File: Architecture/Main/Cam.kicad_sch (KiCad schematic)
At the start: 4 parts, among them J2 Conn_01x02, Q3 NMOS

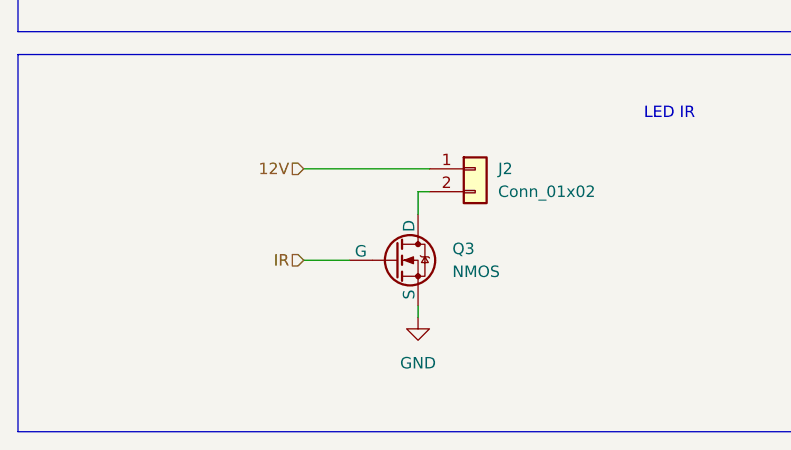
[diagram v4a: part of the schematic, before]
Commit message: Update_She
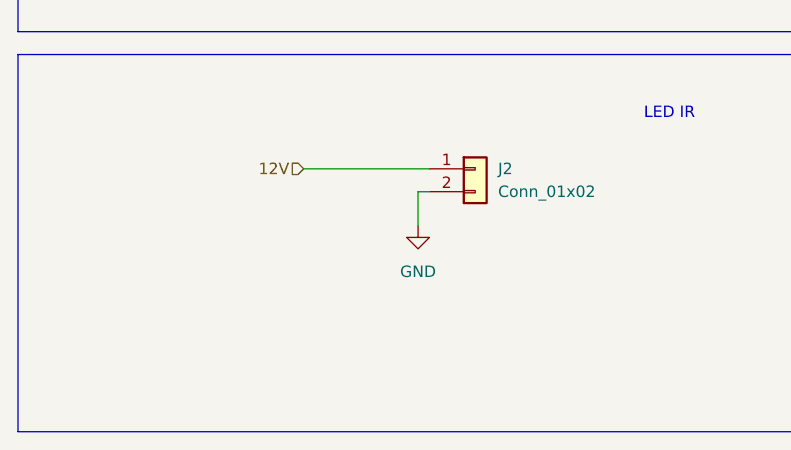
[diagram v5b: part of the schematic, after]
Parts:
- removed Q3: NMOS, symbol Simulation_SPICE:NMOS
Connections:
- net GND: now also J2.2 (Pin_2)
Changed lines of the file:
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@@
 	(wire
 		(pts
-			(xy 171.45 115.57) (xy 176.53 115.57)
-		)
-		(stroke
-			(width 0)
-			(type default)
-		)
-	)
-	(wire
-		(pts
 			(xy 189.23 74.93) (xy 193.04 74.93)
 		)
@@
 	(wire
 		(pts
-			(xy 184.15 110.49) (xy 184.15 107.95)
-		)
-		(stroke
-			(width 0)
-			(type default)
-		)
-	)
-	(wire
-		(pts
 			(xy 172.72 67.31) (xy 176.53 67.31)
 		)
@@
 	(wire
 		(pts
-			(xy 184.15 121.92) (xy 184.15 120.65)
+			(xy 184.15 107.95) (xy 184.15 111.76)
 		)
 		(stroke
@@
 		)
 	)
-	(hierarchical_label "IR"
-		(shape input)
-		(at 171.45 115.57 180)
-		(effects
-			(font
-				(size 1.27 1.27)
-			)
-			(justify right)
-		)
-	)
 	(hierarchical_label "D3"
 		(shape input)
@@
 	)
 	(symbol
-		(lib_id "Simulation_SPICE:NMOS")
-		(at 181.61 115.57 0)
-		(unit 1)
-		(exclude_from_sim no)
-		(in_bom yes)
-		(on_board yes)
-		(dnp no)
-		(fields_autoplaced yes)
-		(property "Reference" "Q3"
-			(at 187.96 114.2999 0)
-			(effects
-				(font
-					(size 1.27 1.27)
-				)
-				(justify left)
-			)
-		)
-		(property "Value" "NMOS"
-			(at 187.96 116.8399 0)
-			(effects
-				(font
-					(size 1.27 1.27)
-				)
-				(justify left)
-			)
-		)
-		(property "Footprint" ""
-			(at 186.69 113.03 0)
-			(effects
-				(font
-					(size 1.27 1.27)
-				)
-				(hide yes)
-			)
-		)
-		(property "Datasheet" "https://ngspice.sourceforge.io/docs/ngspice-html-manual/manual.xhtml#cha_MOSFETs"
-			(at 181.61 128.27 0)
-			(effects
-				(font
-					(size 1.27 1.27)
-				)
-				(hide yes)
-			)
-		)
-		(property "Description" "N-MOSFET transistor, drain/source/gate"
-			(at 181.61 115.57 0)
-			(effects
-				(font
-					(size 1.27 1.27)
-				)
-				(hide yes)
-			)
-		)
-		(property "Sim.Device" "NMOS"
-			(at 181.61 132.715 0)
-			(effects
-				(font
-					(size 1.27 1.27)
-				)
-				(hide yes)
-			)
-		)
-		(property "Sim.Type" "VDMOS"
-			(at 181.61 134.62 0)
-			(effects
-				(font
-					(size 1.27 1.27)
-				)
-				(hide yes)
-			)
-		)
-		(property "Sim.Pins" "1=D 2=G 3=S"
-			(at 181.61 130.81 0)
-			(effects
-				(font
-					(size 1.27 1.27)
-				)
-				(hide yes)
-			)
-		)
-		(pin "3"
-		)
-		(pin "2"
-		)
-		(pin "1"
-		)
-		(instances
-			(project ""
-				(path "/77f264da-4c84-4b0c-9d20-4392731765e6/90e676b5-e192-40ef-8f2d-7a9315f03418"
-					(reference "Q3")
-					(unit 1)
-				)
-			)
-		)
-	)
-	(symbol
 		(lib_id "Device:C")
 		(at 154.94 68.58 0)
@@
 	(symbol
 		(lib_id "power:GND")
-		(at 184.15 121.92 0)
+		(at 184.15 111.76 0)
 		(unit 1)
 		(exclude_from_sim no)
@@
 		(fields_autoplaced yes)
 		(property "Reference" "#PWR024"
-			(at 184.15 128.27 0)
+			(at 184.15 118.11 0)
 			(effects
 				(font
@@
 		)
 		(property "Value" "GND"
-			(at 184.15 127 0)
+			(at 184.15 116.84 0)
 			(effects
 				(font
@@
 		)
 		(property "Footprint" ""
-			(at 184.15 121.92 0)
+			(at 184.15 111.76 0)
 			(effects
 				(font
@@
 		)
 		(property "Datasheet" ""
-			(at 184.15 121.92 0)
+			(at 184.15 111.76 0)
 			(effects
 				(font
@@
 		)
 		(property "Description" "Power symbol creates a global label with name \"GND\" , ground"
-			(at 184.15 121.92 0)
+			(at 184.15 111.76 0)
 			(effects
 				(font
